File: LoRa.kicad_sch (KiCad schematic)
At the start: 26 parts, among them J10 Conn_Coaxial, J20 Conn_01x01, J21 Conn_01x01, J22 Conn_01x01, J23 Conn_01x01, J24 Conn_01x01, J25 Conn_01x01, J26 Conn_01x01, J6 Conn_Coaxial, U1 NCV8170AXV300T2G, U2 Quectel_L96, U5 E22-900M22S

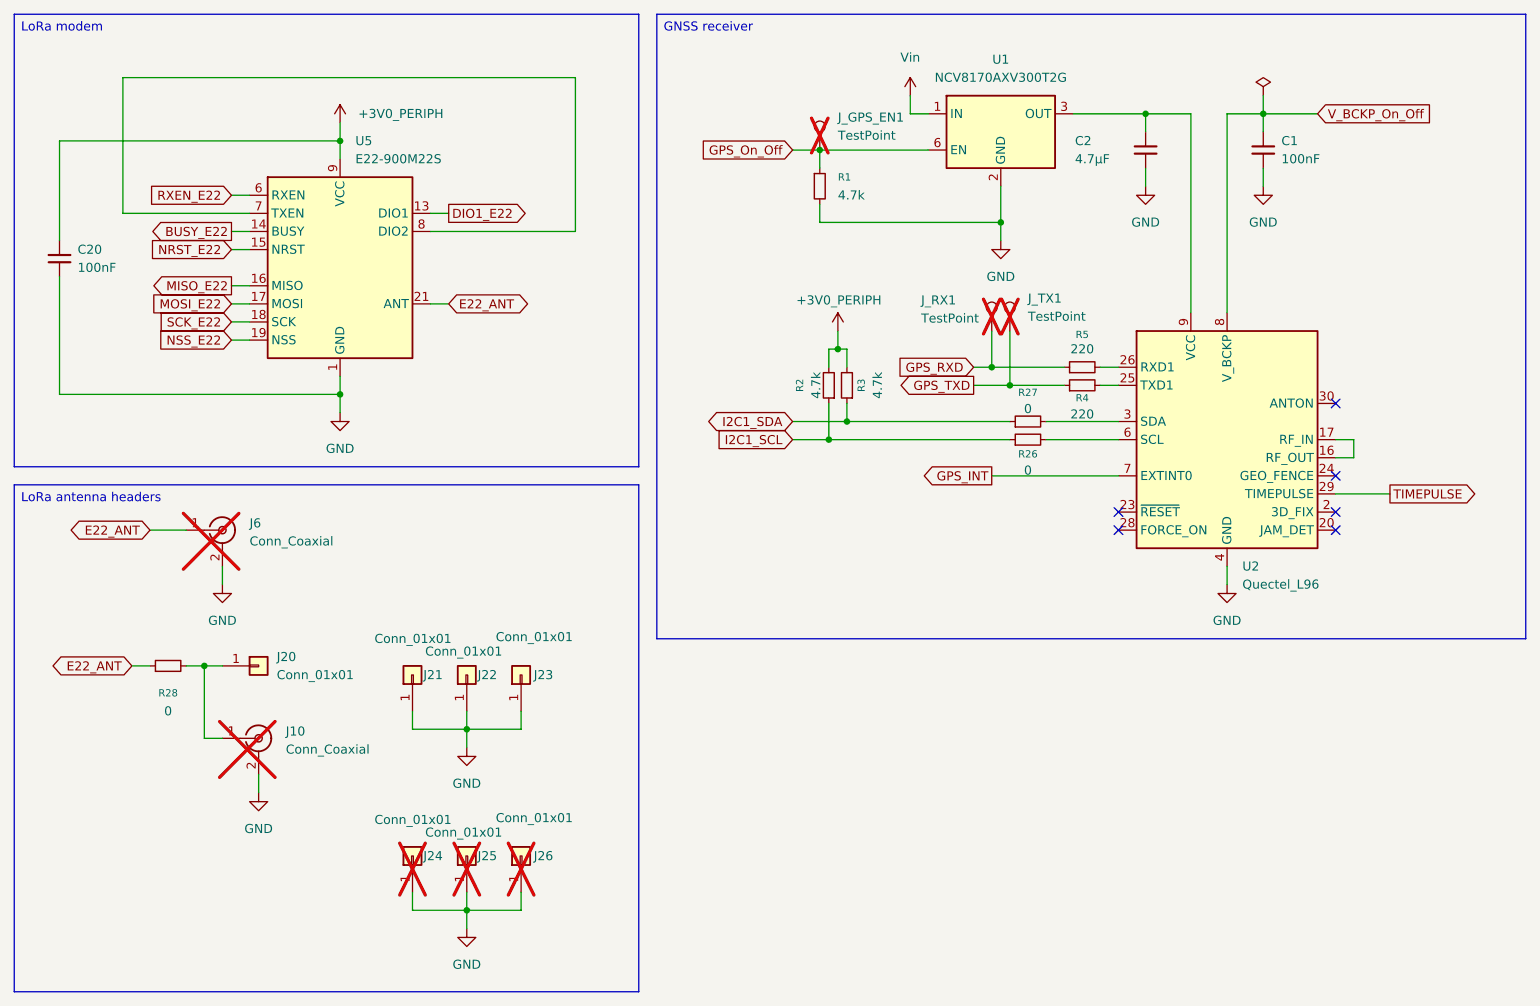
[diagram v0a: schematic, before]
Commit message: WIP: BOM
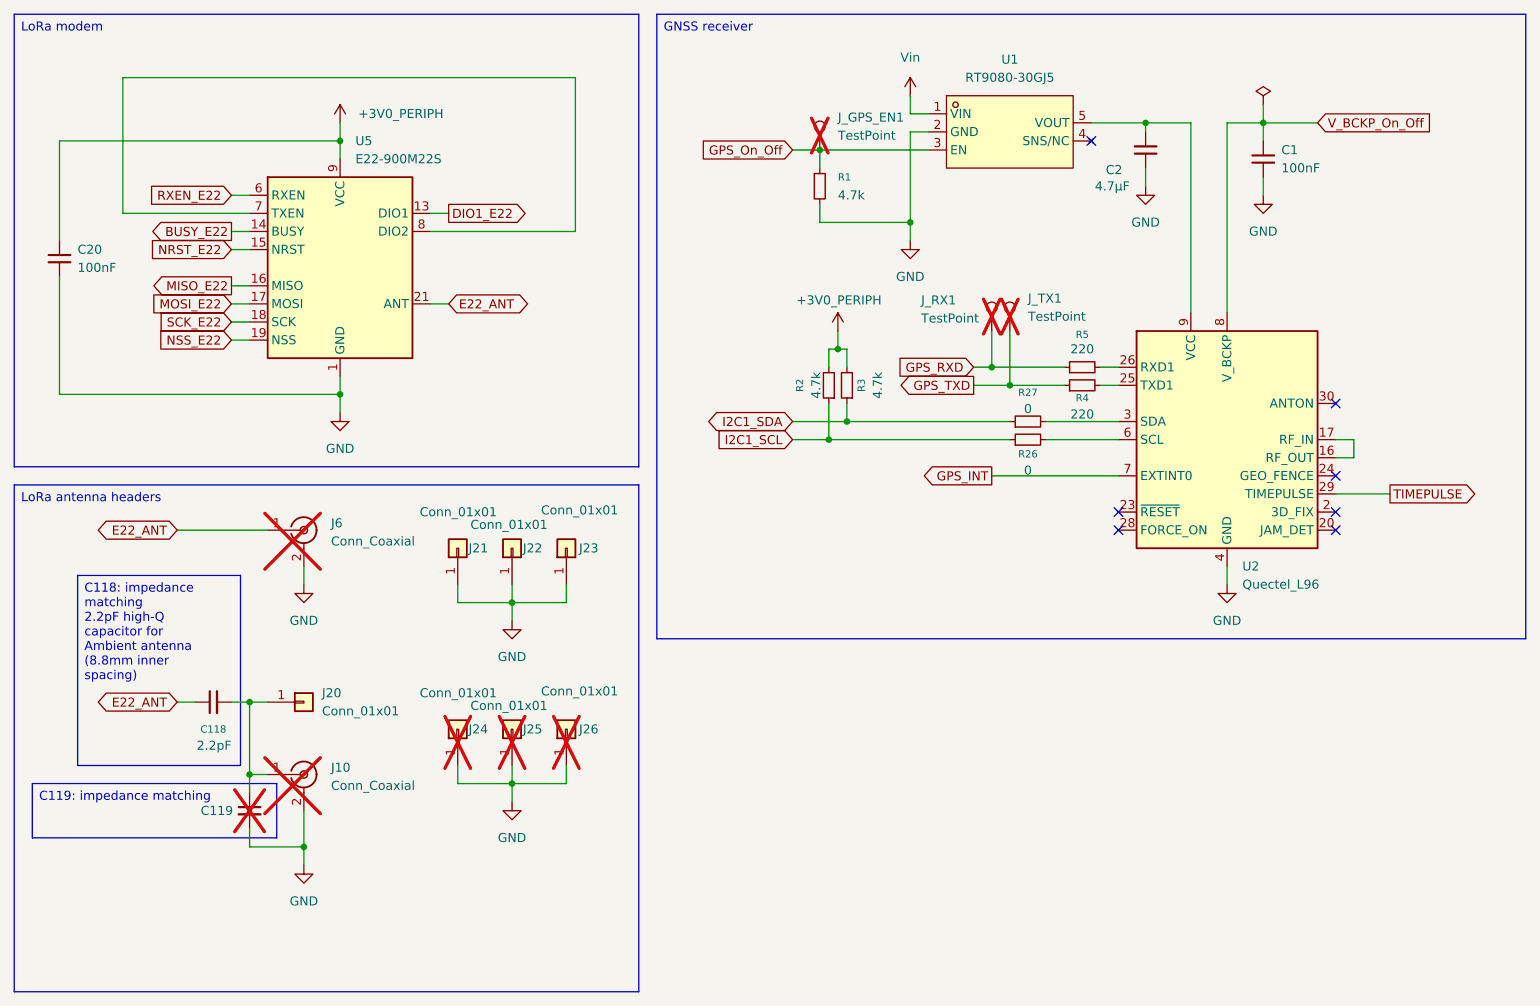
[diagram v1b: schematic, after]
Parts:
- removed R28: 0, Resistor_SMD:R_0805_2012Metric, symbol Device:R_Small
- removed U1: NCV8170AXV300T2G, Package_TO_SOT_SMD:SOT-563, symbol Onsemi_NCV8170:NCV8170AXV300T2G
- added C118: 2.2pF, Capacitor_SMD:C_0402_1005Metric, symbol Device:C_Small
- added C119: (no value), Capacitor_SMD:C_0402_1005Metric, symbol Device:C_Small
- added U1: RT9080-30GJ5, Package_TO_SOT_SMD:TSOT-23-5, symbol RT9080-30GJ5:RT9080-30GJ5
- C1, C20: LCSC (none) -> C1525
- C2: LCSC (none) -> C23733
- J10: LCSC (none) -> C88373
- J20, J21, J22, J23, J24, J25, J26: LCSC (none) -> C25503131
- J6: LCSC (none) -> C88373; now left out of the parts list
- R1, R2, R3: LCSC (none) -> C25900
- R26, R27: LCSC (none) -> C17168
- R4, R5: LCSC (none) -> C25091
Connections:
- net E22_ANT: now also C118.1
- net GND: now also C119.2, U1.2 (GND)
- net GPS_On_Off: now also U1.3 (EN)
- net Vin: now also U1.1 (VIN)
- net at J10.1 (In), J20.1 (Pin_1): now also C118.2, C119.1
- net at C2.1, U2.9 (VCC): now also U1.5 (VOUT)
- no-connect marks 6 -> 7
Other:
- moved on the sheet: C1, J10, J20, J21, J22, J23, J24, J25, J26, J6

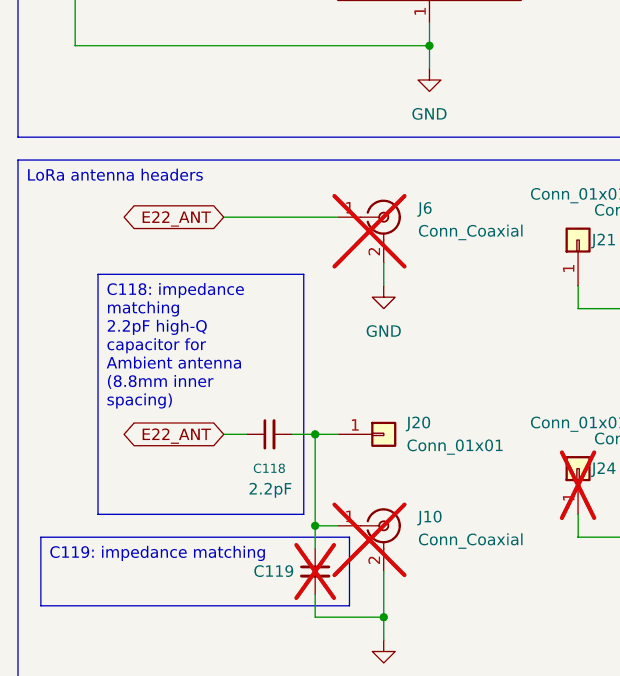
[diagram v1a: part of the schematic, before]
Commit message: WIP: omit some components and perform initial rough placement on PCB
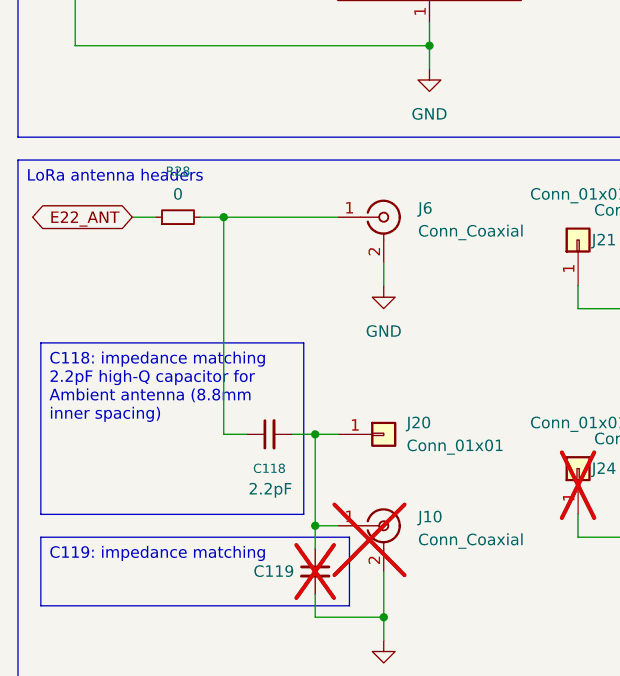
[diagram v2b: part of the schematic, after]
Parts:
- added R28: 0, Resistor_SMD:R_0402_1005Metric, symbol Device:R_Small
- J10: now left out of the parts list
- J6: now fitted; now in the parts list
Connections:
- net E22_ANT: now also R28.1; no longer C118.1, J6.1 (In)
- new net: C118.1, J6.1 (In), R28.2
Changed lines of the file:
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@@
 	(text_box "C118: impedance matching\n2.2pF high-Q capacitor for Ambient antenna (8.8mm inner spacing)"
 		(exclude_from_sim no)
-		(at 39.37 118.11 0)
-		(size 22.86 26.67)
+		(at 33.02 125.73 0)
+		(size 29.21 19.05)
 		(margins 0.9525 0.9525 0.9525 0.9525)
 		(stroke
@@
 	)
 	(junction
+		(at 53.34 111.76)
+		(diameter 0)
+		(color 0 0 0 0)
+	)
+	(junction
 		(at 147.32 96.52)
 		(diameter 0)
@@
 	(wire
 		(pts
-			(xy 53.34 135.89) (xy 55.88 135.89)
-		)
-		(stroke
-			(width 0)
-			(type default)
-		)
-	)
-	(wire
-		(pts
 			(xy 139.7 58.42) (xy 143.51 58.42)
 		)
@@
 	(wire
 		(pts
-			(xy 53.34 111.76) (xy 66.04 111.76)
+			(xy 43.18 111.76) (xy 45.72 111.76)
 		)
 		(stroke
@@
 	(wire
 		(pts
+			(xy 53.34 111.76) (xy 66.04 111.76)
+		)
+		(stroke
+			(width 0)
+			(type default)
+		)
+	)
+	(wire
+		(pts
 			(xy 156.21 55.88) (xy 156.21 68.58)
 		)
@@
 	(wire
 		(pts
+			(xy 53.34 111.76) (xy 53.34 135.89)
+		)
+		(stroke
+			(width 0)
+			(type default)
+		)
+	)
+	(wire
+		(pts
 			(xy 71.12 158.75) (xy 71.12 156.21)
 		)
@@
 	(wire
 		(pts
+			(xy 53.34 135.89) (xy 55.88 135.89)
+		)
+		(stroke
+			(width 0)
+			(type default)
+		)
+	)
+	(wire
+		(pts
+			(xy 50.8 111.76) (xy 53.34 111.76)
+		)
+		(stroke
+			(width 0)
+			(type default)
+		)
+	)
+	(wire
+		(pts
 			(xy 60.96 82.55) (xy 63.5 82.55)
 		)
@@
 	(global_label "E22_ANT"
 		(shape bidirectional)
-		(at 53.34 111.76 180)
+		(at 43.18 111.76 180)
 		(fields_autoplaced yes)
 		(effects
@@
 		)
 		(property "Intersheetrefs" "${INTERSHEET_REFS}"
-			(at 41.3212 111.76 0)
+			(at 31.1612 111.76 0)
 			(hide yes)
 			(show_name no)
@@
 		)
 	)
-	(global_label "E22_ANT"
-		(shape bidirectional)
-		(at 53.34 135.89 180)
-		(fields_autoplaced yes)
-		(effects
-			(font
-				(size 1.27 1.27)
-			)
-			(justify right)
-		)
-		(property "Intersheetrefs" "${INTERSHEET_REFS}"
-			(at 41.3212 135.89 0)
-			(hide yes)
-			(show_name no)
-			(do_not_autoplace no)
-			(effects
-				(font
-					(size 1.27 1.27)
-				)
-				(justify right)
-			)
-		)
-	)
 	(global_label "NSS_E22"
 		(shape input)
@@
 		(body_style 1)
 		(exclude_from_sim no)
-		(in_bom no)
-		(on_board no)
-		(in_pos_files no)
-		(dnp yes)
+		(in_bom yes)
+		(on_board yes)
+		(in_pos_files yes)
+		(dnp no)
 		(fields_autoplaced yes)
 		(property "Reference" "J6"
@@
 		(body_style 1)
 		(exclude_from_sim no)
-		(in_bom yes)
-		(on_board yes)
-		(in_pos_files yes)
+		(in_bom no)
+		(on_board no)
+		(in_pos_files no)
 		(dnp yes)
 		(fields_autoplaced yes)
@@
 					(unit 1)
 				)
+			)
+		)
+	)
+	(symbol
+		(lib_id "Device:R_Small")
+		(at 48.26 111.76 90)
+		(unit 1)
+		(body_style 1)
+		(exclude_from_sim no)
+		(in_bom yes)
+		(on_board yes)
+		(in_pos_files yes)
+		(dnp no)
+		(fields_autoplaced yes)
+		(property "Reference" "R28"
+			(at 48.26 106.68 90)
+			(show_name no)
+			(do_not_autoplace no)
+			(effects
+				(font
+					(size 1.016 1.016)
+				)
+			)
+		)
+		(property "Value" "0"
+			(at 48.26 109.22 90)
+			(show_name no)
+			(do_not_autoplace no)
+			(effects
+				(font
+					(size 1.27 1.27)
+				)
+			)
+		)
+		(property "Footprint" "Resistor_SMD:R_0402_1005Metric"
+			(at 48.26 111.76 0)
+			(hide yes)
+			(show_name no)
+			(do_not_autoplace no)
+			(effects
+				(font
+					(size 1.27 1.27)
+				)
+			)
+		)
+		(property "Datasheet" ""
+			(at 48.26 111.76 0)
+			(hide yes)
+			(show_name no)
+			(do_not_autoplace no)
+			(effects
+				(font
+					(size 1.27 1.27)
+				)
+			)
+		)
+		(property "Description" "Resistor, small symbol"
+			(at 48.26 111.76 0)
+			(hide yes)
+			(show_name no)
+			(do_not_autoplace no)
+			(effects
+				(font
+					(size 1.27 1.27)
+				)
+			)
+		)
+		(property "LCSC" "C17168"
+			(at 48.26 111.76 90)
+			(hide yes)
+			(show_name no)
+			(do_not_autoplace no)
+			(effects
+				(font
+					(size 1.27 1.27)
+				)
+			)
+		)
+		(pin "1"
+		)
+		(pin "2"
+		)
+		(instances
+			(project "uca-dkaiot2-kicad"
+				(path "/13b7de53-ecff-4b32-b513-b5b471d022a3/32a654bf-d623-4518-9392-f2b212dc4f8b"
+					(reference "R28")
+					(unit 1)
+				)

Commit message: Finish routing + silkscreen placement
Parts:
- J6: footprint Connector_Coaxial:U.FL_Hirose_U.FL-R-SMT-1_Vertical -> U.FL_Hirose_No_Keepout:U.FL_Hirose_U.FL-R-SMT-1_Vertical_No_Keepout
- U2: FT Position Offset (none) -> 0.508,0.0
- U5: FT Position Offset (none) -> 0.0,-0.508
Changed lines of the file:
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@@
 			)
 		)
-		(property "Footprint" "Connector_Coaxial:U.FL_Hirose_U.FL-R-SMT-1_Vertical"
+		(property "Footprint" "U.FL_Hirose_No_Keepout:U.FL_Hirose_U.FL-R-SMT-1_Vertical_No_Keepout"
 			(at 71.12 111.76 0)
 			(hide yes)
@@
 			)
 		)
+		(property "FT Position Offset" "0.508,0.0"
+			(at 200.66 99.06 0)
+			(hide yes)
+			(show_name no)
+			(do_not_autoplace no)
+			(effects
+				(font
+					(size 1.27 1.27)
+				)
+			)
+		)
 		(pin "3"
 		)
@@
 			(at 76.2 74.93 0)
 			(hide yes)
+			(show_name no)
+			(do_not_autoplace no)
+			(effects
+				(font
+					(size 1.27 1.27)
+				)
+			)
+		)
+		(property "FT Position Offset" "0.0,-0.508"
+			(at 76.2 74.93 0)
+			(hide yes)

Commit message: JLCPCB offsets and small fixes
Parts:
- J6: FT Position Offset (none) -> -0.508,0.0
- U2: FT Position Offset 0.508,0.0 -> 0,0.508
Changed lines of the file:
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@@
+			)
+		)
+		(property "FT Position Offset" "-0.508,0.0"
+			(at 71.12 111.76 0)
+			(hide yes)
+			(show_name no)
+			(do_not_autoplace no)
+			(effects
+				(font
+					(size 1.27 1.27)
+				)
 			)
 		)
@@
 			)
 		)
-		(property "FT Position Offset" "0.508,0.0"
+		(property "FT Position Offset" "0,0.508"
 			(at 200.66 99.06 0)
 			(hide yes)
